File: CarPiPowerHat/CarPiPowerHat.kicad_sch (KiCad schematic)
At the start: 14 parts, among them J3 40HAT, J4 Conn_02x03_Counter_Clockwise, J9 Conn_01x04, U2 CAT24C32

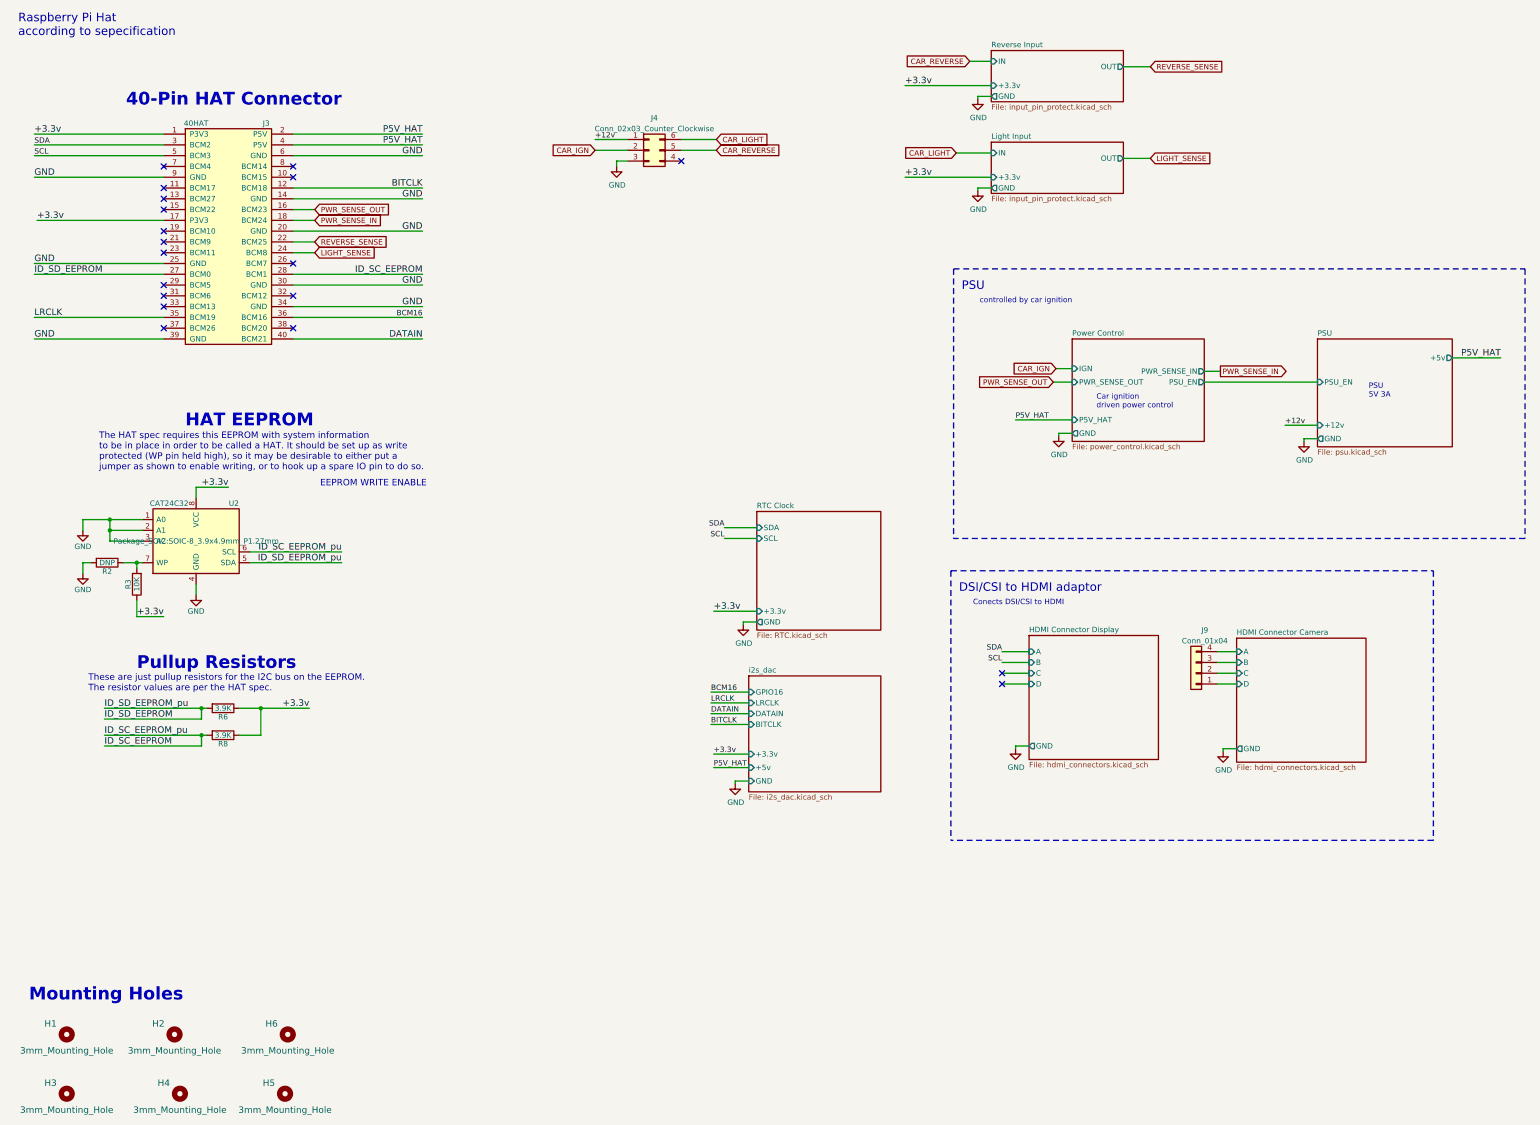
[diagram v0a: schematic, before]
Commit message: Everything routed, DRC ok
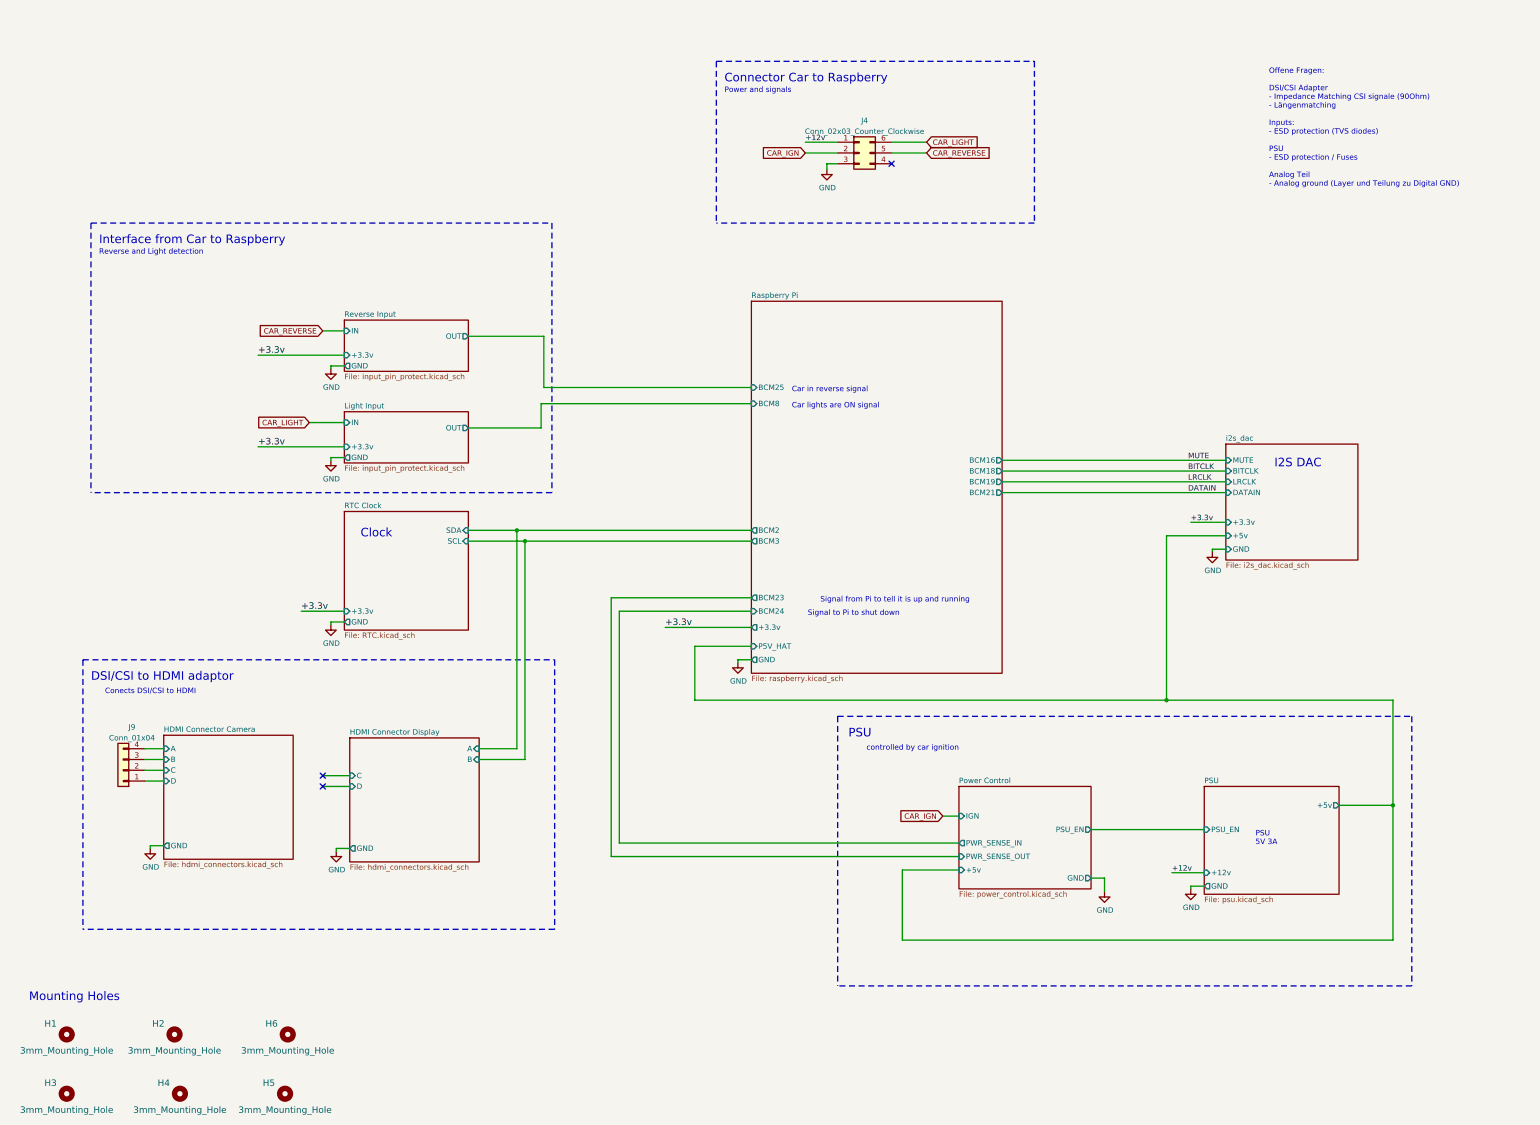
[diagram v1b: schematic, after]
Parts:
- removed J3: 40HAT, Connector_PinSocket_2.54mm:PinSocket_2x20_P2.54mm_Vertical, symbol CarPiPowerHat:OX40HAT
- removed R2: DNP, project_footprints:R_0603_1608Metric_Pad0.84x1.00mm_HandSolder, symbol Device:R
- removed R3: 10K, Resistor_SMD:R_0603_1608Metric, symbol Device:R
- removed R6, R8: 3.9K, Resistor_SMD:R_0603_1608Metric, symbol Device:R
- removed U2: CAT24C32, Package_SOIC:SOIC-8_3.9x4.9mm_P1.27mm, symbol CarPiPowerHat:CAT24C32
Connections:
- no-connect marks 19 -> 3
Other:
- added sheet Raspberry Pi (raspberry.kicad_sch)
- sheet Power Control ports: added +5v; removed P5V_HAT
- sheet i2s_dac ports: added MUTE; removed GPIO16
- note added: "Car in reverse signal"
- note added: "Car lights are ON signal"
- note added: "Clock"
- note added: "Connector Car to Raspberry"
- note added: "I2S DAC"
- note added: "Interface from Car to Raspberry"
- note added: "Offene Fragen: DSI/CSI Adapter - Impedance Matching CSI signale (90Ohm) - Längenmatching Inputs: - ESD protection (TVS diodes) PSU - ESD protection / Fuses Analog Teil - Analog ground (Layer und Teilung zu Digital GND)"
- note added: "Power and signals"
- note added: "Reverse and Light detection"
- note added: "Signal from Pi to tell it is up and running"
- note added: "Signal to Pi to shut down"
- note removed: "40-Pin HAT Connector"
- note removed: "Car ignition driven power control"
- note removed: "EEPROM WRITE ENABLE"
- note removed: "HAT EEPROM"
- note removed: "Pullup Resistors"
- note removed: "Raspberry Pi Hat according to sepecification"
- note removed: "The HAT spec requires this EEPROM with system information to be in place in order to be called a HAT. It should be set up as write protected (WP pin held high), so it may be desirable to either put a jumper as shown to enable writing, or to hook up a spare IO pin to do so."
- note removed: "These are just pullup resistors for the I2C bus on the EEPROM. The resistor values are per the HAT spec."
- moved on the sheet: J4, J9
